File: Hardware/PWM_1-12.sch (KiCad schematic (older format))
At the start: 0 parts

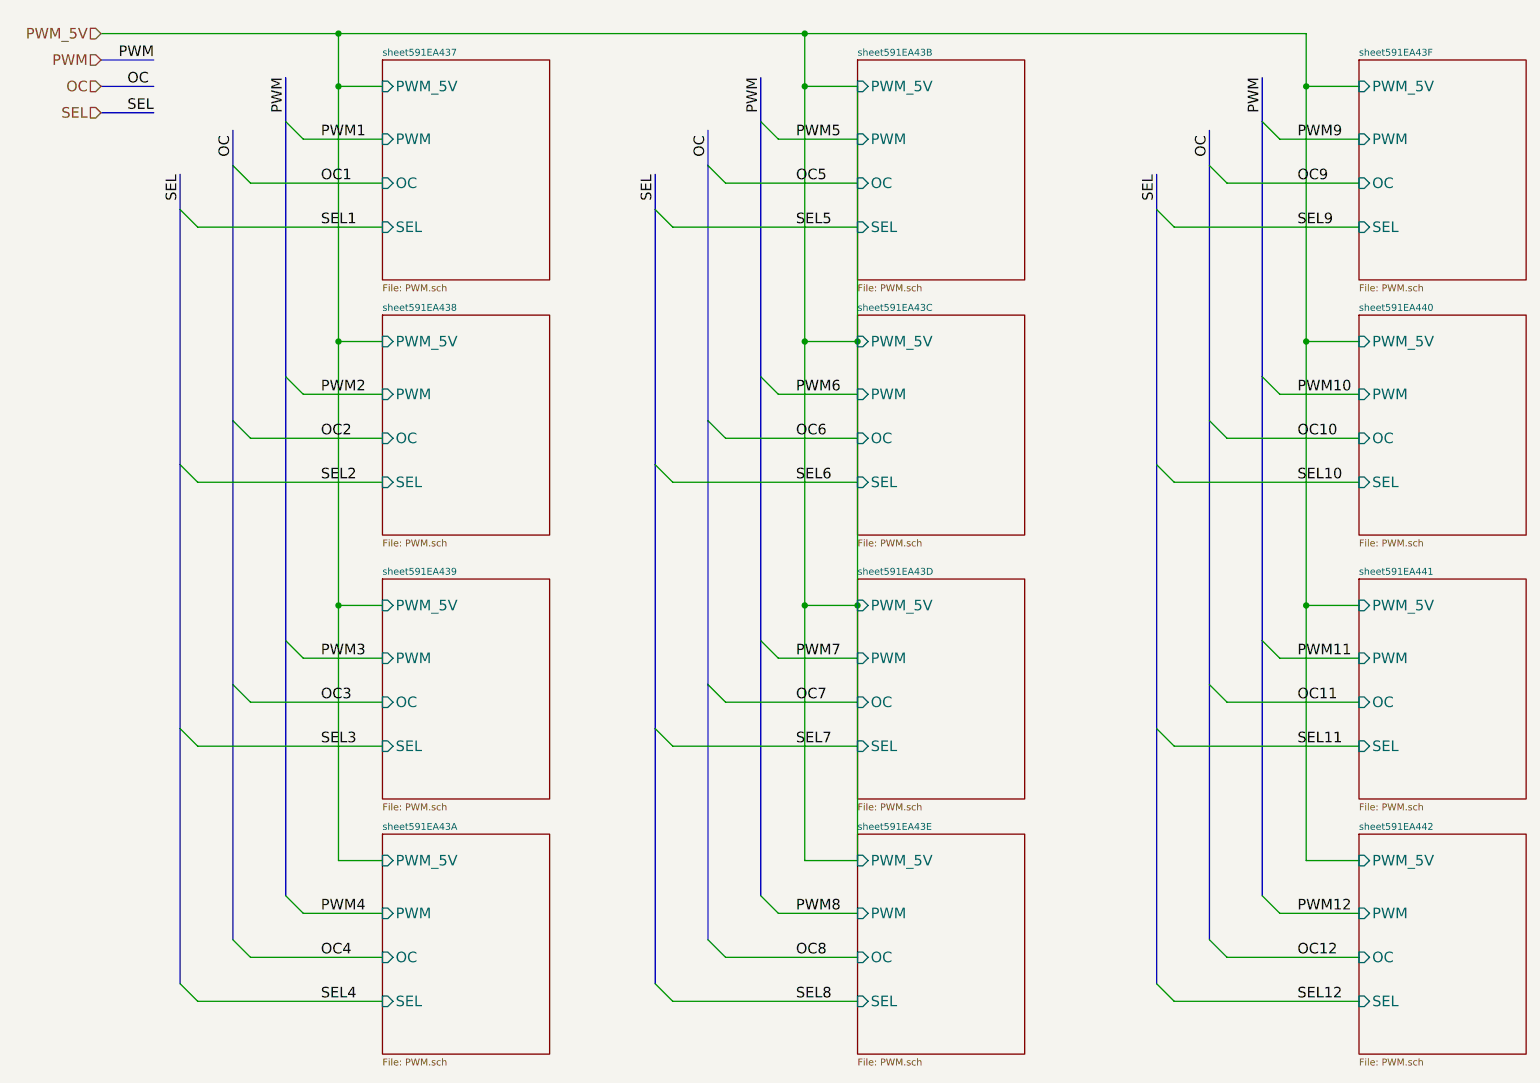
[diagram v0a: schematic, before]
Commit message: ALL THE POWER
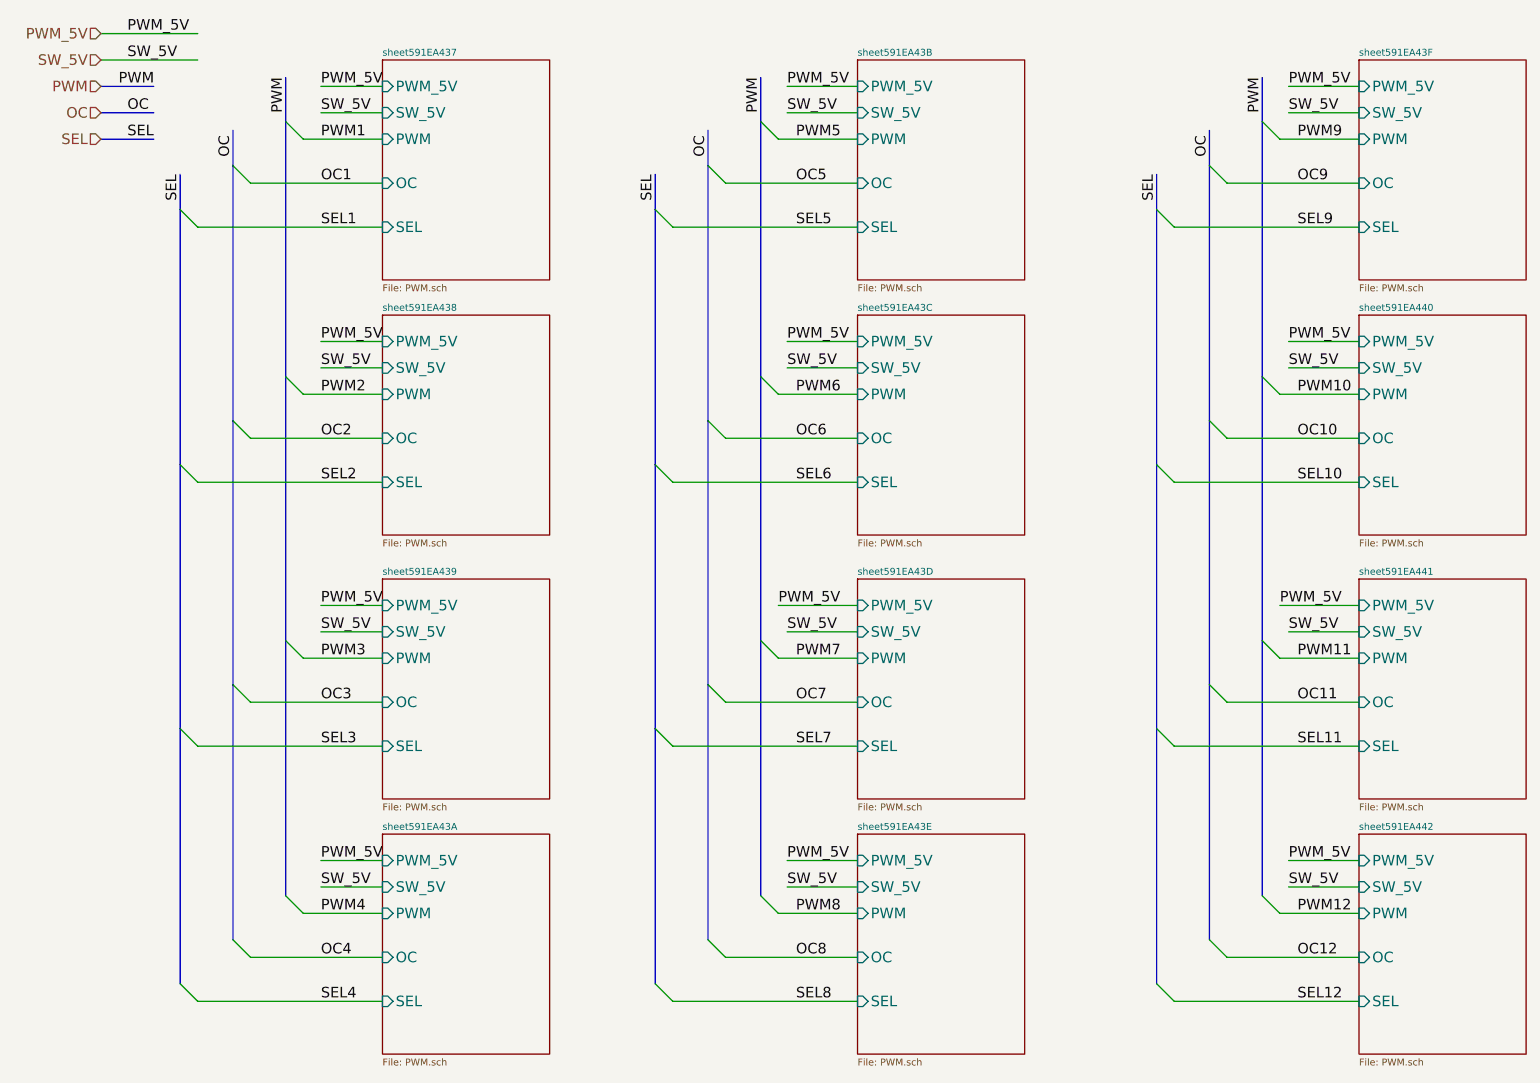
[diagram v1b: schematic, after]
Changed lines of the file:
@@
 LIBS:valves
 LIBS:WARG
+LIBS:ZeroPilot-cache
 EELAYER 25 0
 EELAYER END
 $Descr A4 11693 8268
 encoding utf-8
-Sheet 2 14
+Sheet 2 15
 Title "PWM 1-12"
 Date "2017-05-13"
@@
 F4 "PWM" I L 2700 1250 60
 F5 "OC" I L 2700 1500 60
+F6 "SW_5V" I L 2700 1100 60
 $EndSheet
 $Sheet
@@
 F4 "PWM" I L 2700 2700 60
 F5 "OC" I L 2700 2950 60
+F6 "SW_5V" I L 2700 2550 60
 $EndSheet
 $Sheet
@@
 F4 "PWM" I L 2700 4200 60
 F5 "OC" I L 2700 4450 60
+F6 "SW_5V" I L 2700 4050 60
 $EndSheet
 $Sheet
@@
 F4 "PWM" I L 2700 5650 60
 F5 "OC" I L 2700 5900 60
+F6 "SW_5V" I L 2700 5500 60
 $EndSheet
 $Sheet
@@
 F4 "PWM" I L 5400 1250 60
 F5 "OC" I L 5400 1500 60
+F6 "SW_5V" I L 5400 1100 60
 $EndSheet
 $Sheet
@@
 F4 "PWM" I L 5400 2700 60
 F5 "OC" I L 5400 2950 60
+F6 "SW_5V" I L 5400 2550 60
 $EndSheet
 $Sheet
@@
 F4 "PWM" I L 5400 4200 60
 F5 "OC" I L 5400 4450 60
+F6 "SW_5V" I L 5400 4050 60
 $EndSheet
 $Sheet
@@
 F4 "PWM" I L 5400 5650 60
 F5 "OC" I L 5400 5900 60
+F6 "SW_5V" I L 5400 5500 60
 $EndSheet
 $Sheet
@@
 F4 "PWM" I L 8250 1250 60
 F5 "OC" I L 8250 1500 60
+F6 "SW_5V" I L 8250 1100 60
 $EndSheet
 $Sheet
@@
 F4 "PWM" I L 8250 2700 60
 F5 "OC" I L 8250 2950 60
+F6 "SW_5V" I L 8250 2550 60
 $EndSheet
 $Sheet
@@
 F4 "PWM" I L 8250 4200 60
 F5 "OC" I L 8250 4450 60
+F6 "SW_5V" I L 8250 4050 60
 $EndSheet
 $Sheet
@@
 F4 "PWM" I L 8250 5650 60
 F5 "OC" I L 8250 5900 60
+F6 "SW_5V" I L 8250 5500 60
 $EndSheet
 Entry Wire Line
@@
 SEL12
 Wire Wire Line
-	2700 950  2450 950
-Wire Wire Line
-	2450 650  2450 650
-Wire Wire Line
-	2450 650  2450 950
-Wire Wire Line
-	2450 950  2450 2400
-Wire Wire Line
-	2450 2400 2450 3900
-Wire Wire Line
-	2450 3900 2450 5350
-Wire Wire Line
-	2450 5350 2700 5350
-Wire Wire Line
-	5400 950  5400 2400
-Wire Wire Line
-	5400 2400 5400 3900
-Wire Wire Line
-	5400 3900 5400 5350
-Wire Wire Line
-	5400 950  5100 950
-Wire Wire Line
-	5100 650  5100 950
-Wire Wire Line
-	5100 950  5100 2400
-Wire Wire Line
-	5100 2400 5100 3900
-Wire Wire Line
-	5100 3900 5100 5350
-Wire Wire Line
-	5100 5350 5400 5350
-Wire Wire Line
-	5400 3900 5100 3900
-Connection ~ 5100 3900
-Connection ~ 5400 3900
-Wire Wire Line
-	5400 2400 5100 2400
-Connection ~ 5100 2400
-Connection ~ 5400 2400
-Wire Wire Line
-	8250 950  7950 950
-Wire Wire Line
-	7950 650  7950 950
-Wire Wire Line
-	7950 950  7950 2400
-Wire Wire Line
-	7950 2400 7950 3900
-Wire Wire Line
-	7950 3900 7950 5350
-Wire Wire Line
-	7950 5350 8250 5350
-Wire Wire Line
-	8250 3900 7950 3900
-Connection ~ 7950 3900
-Wire Wire Line
-	8250 2400 7950 2400
-Connection ~ 7950 2400
-Wire Wire Line
-	2450 650  5100 650
-Wire Wire Line
-	5100 650  7950 650
-Connection ~ 2450 950
-Connection ~ 7950 950
-Connection ~ 5100 650
-Connection ~ 5100 950
+	2700 950  2350 950
+Wire Wire Line
+	1100 650  1650 650
+Wire Wire Line
+	2350 5350 2700 5350
+Wire Wire Line
+	5400 950  5000 950
+Wire Wire Line
+	5000 5350 5400 5350
+Wire Wire Line
+	5400 3900 4950 3900
+Wire Wire Line
+	5400 2400 5000 2400
+Wire Wire Line
+	8250 950  7850 950
+Wire Wire Line
+	7850 5350 8250 5350
+Wire Wire Line
+	8250 3900 7800 3900
+Wire Wire Line
+	8250 2400 7850 2400
 Wire Bus Line
 	2150 900  2150 1150
@@
 	2250 5650 2700 5650
 Wire Wire Line
-	2700 3900 2450 3900
-Connection ~ 2450 3900
+	2700 3900 2350 3900
 Wire Wire Line
 	2250 4200 2700 4200
 Wire Wire Line
-	2700 2400 2450 2400
-Connection ~ 2450 2400
+	2700 2400 2350 2400
 Wire Wire Line
 	2700 2700 2250 2700
@@
 Wire Wire Line
 	7200 1750 8250 1750
+Text HLabel 1100 1100 0    60   Input ~ 0
+OC
 Text HLabel 1100 950  0    60   Input ~ 0
-OC
-Text HLabel 1100 800  0    60   Input ~ 0
 PWM
-Text HLabel 1100 1100 0    60   Input ~ 0
+Text HLabel 1100 1250 0    60   Input ~ 0
 SEL
 Text HLabel 1100 650  0    60   Input ~ 0
 PWM_5V
-Wire Wire Line
-	2450 650  1100 650
-Connection ~ 2450 650
-Wire Bus Line
-	1100 800  1400 800
 Wire Bus Line
 	1100 950  1400 950
 Wire Bus Line
 	1100 1100 1400 1100
-Text Label 1200 800  0    60   ~ 0
+Wire Bus Line
+	1100 1250 1400 1250
+Text Label 1200 950  0    60   ~ 0
 PWM
-Text Label 1250 950  0    60   ~ 0
+Text Label 1250 1100 0    60   ~ 0
 OC
-Text Label 1250 1100 0    60   ~ 0
+Text Label 1250 1250 0    60   ~ 0
 SEL
+Text Label 2350 950  0    60   ~ 0
+PWM_5V
+Text Label 2350 2400 0    60   ~ 0
+PWM_5V
+Text Label 2350 3900 0    60   ~ 0
+PWM_5V
+Text Label 2350 5350 0    60   ~ 0
+PWM_5V
+Text Label 5000 950  0    60   ~ 0
+PWM_5V
+Text Label 5000 2400 0    60   ~ 0
+PWM_5V
+Text Label 4950 3900 0    60   ~ 0
+PWM_5V
+Text Label 5000 5350 0    60   ~ 0
+PWM_5V
+Text Label 7850 950  0    60   ~ 0
+PWM_5V
+Text Label 7850 2400 0    60   ~ 0
+PWM_5V
+Text Label 7800 3900 0    60   ~ 0
+PWM_5V
+Text Label 7850 5350 0    60   ~ 0
+PWM_5V
+Text Label 1250 650  0    60   ~ 0
+PWM_5V
+Wire Wire Line
+	2700 1100 2350 1100
+Wire Wire Line
+	2350 2550 2700 2550
+Wire Wire Line
+	2350 4050 2700 4050
+Wire Wire Line
+	2700 5500 2350 5500
+Wire Wire Line
+	5000 5500 5400 5500
+Wire Wire Line
+	5000 4050 5400 4050
+Wire Wire Line
+	5000 2550 5400 2550
+Wire Wire Line
+	7850 5500 8250 5500
+Wire Wire Line
+	7850 4050 8250 4050
+Wire Wire Line
+	7850 2550 8250 2550
+Wire Wire Line
+	7850 1100 8250 1100
+Wire Wire Line
+	5000 1100 5400 1100
+Text Label 7850 1100 0    60   ~ 0
+SW_5V
+Text Label 7850 2550 0    60   ~ 0
+SW_5V
+Text Label 7850 4050 0    60   ~ 0
+SW_5V
+Text Label 5000 4050 0    60   ~ 0
+SW_5V
+Text Label 5000 2550 0    60   ~ 0
+SW_5V
+Text Label 5000 1100 0    60   ~ 0
+SW_5V
+Text Label 7850 5500 0    60   ~ 0
+SW_5V
+Text Label 5000 5500 0    60   ~ 0
+SW_5V
+Text Label 2350 5500 0    60   ~ 0
+SW_5V
+Text Label 2350 4050 0    60   ~ 0
+SW_5V
+Text Label 2350 2550 0    60   ~ 0
+SW_5V
+Text Label 2350 1100 0    60   ~ 0
+SW_5V
+Text HLabel 1100 800  0    60   Input ~ 0
+SW_5V
+Wire Wire Line
+	1100 800  1650 800
+Text Label 1250 800  0    60   ~ 0
+SW_5V
 $EndSCHEMATC
